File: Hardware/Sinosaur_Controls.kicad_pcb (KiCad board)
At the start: 2 copper layers, 60 x 110 mm, 35 parts, among them J1 Conn_01x12_Male, J10 Sine1InvOut, J11 FM2Out, J12 FM3Out, J13 SwellOut, J14 ClockIn, J2 Conn_01x12_Male, J3 Conn_01x16_Male, J4 Conn_01x16_Male, J5 Sine1Out, J6 Sine2Out, J7 Sine3Out, J8 RampOut, J9 GateIn

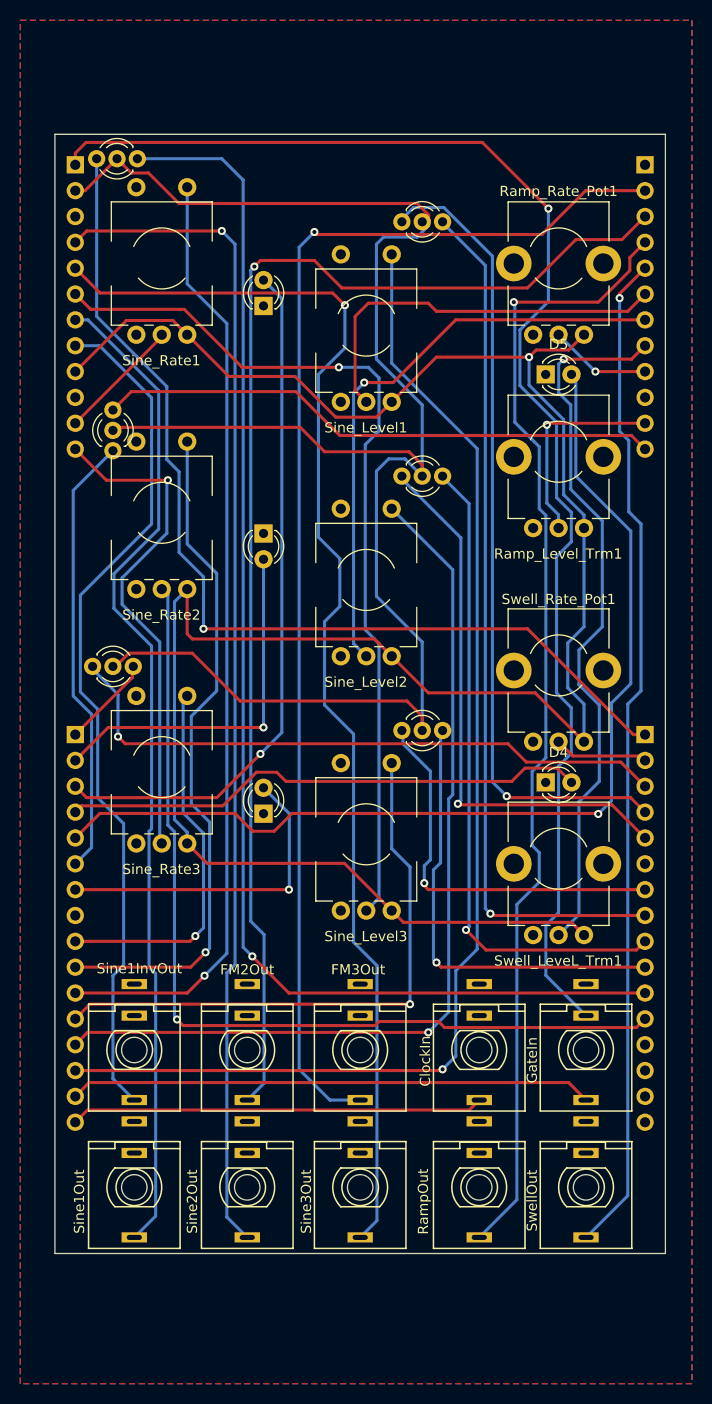
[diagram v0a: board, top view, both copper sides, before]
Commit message: Gerber production
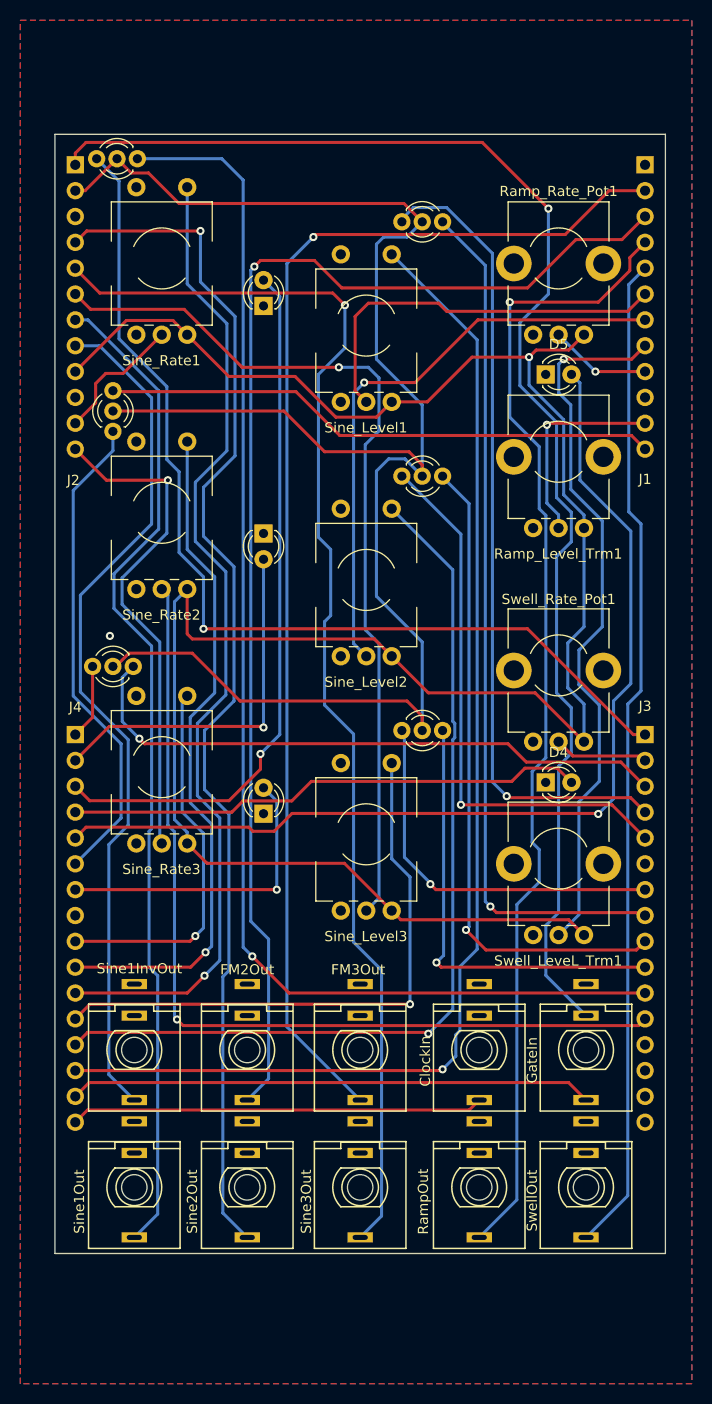
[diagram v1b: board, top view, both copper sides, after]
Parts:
- moved D8 1.90 mm to (105.7, 77.2)
- turned D10 to 180 degrees
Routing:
- net /Sine1_Rate_Btn: track 93.4 -> 97.7 mm
- net /Sine2_Ramp_Rate_LED: track 43.6 -> 47.9 mm
- net /Sine2_Out: track 115.5 -> 119.1 mm
- net /Sine3_Ramp_Rate_LED: track 61.7 -> 59.9 mm
- net /Sine3_LED: track 32.1 -> 30.3 mm
- net /Sine3_Swell_Rate_LED: track 9.02 -> 7.40 mm
- net +3.3V: track 170.6 -> 169.3 mm
- net /Sine1_Rate: track 12.2 -> 13.4 mm
- net /FM3_Out: track 124.6 -> 123.4 mm
- net /Ramp_LED: track 100.8 -> 99.7 mm
- net /Sine1_LED: track 68.6 -> 69.6 mm
- net /Sine3_Ramp_Lvl_LED: track 38.5 -> 37.6 mm
- net /Swell_Out: track 99.4 -> 98.7 mm, vias 1 -> 0
- net /Swell_LED: track 51.9 -> 51.1 mm
- net /Sine2_Swell_Rate_LED: track 55.4 -> 54.7 mm
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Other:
- board text added: "J1"
- board text added: "J2"
- board text added: "J3"
- board text added: "J4"
- board text added: "Mountjoy Modular 2024 Sinosaur Controls v1.0"
